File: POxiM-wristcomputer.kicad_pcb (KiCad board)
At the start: 4 copper layers, 38.1 x 22.6 mm, 58 parts, among them J1 USB_B_Micro, J2 AudioJack4_Ground, U1 LM321, U2 STM8S003F3P

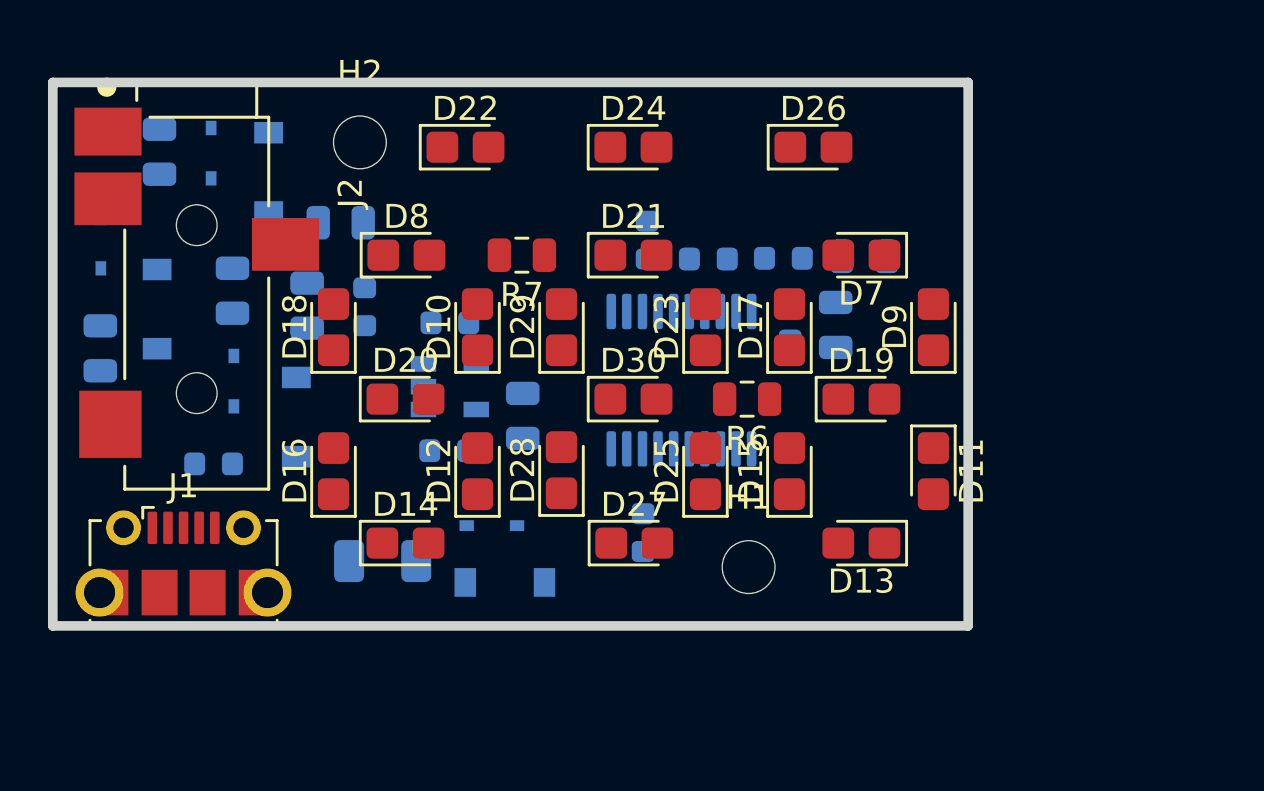
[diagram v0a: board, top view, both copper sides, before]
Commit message: big chungus
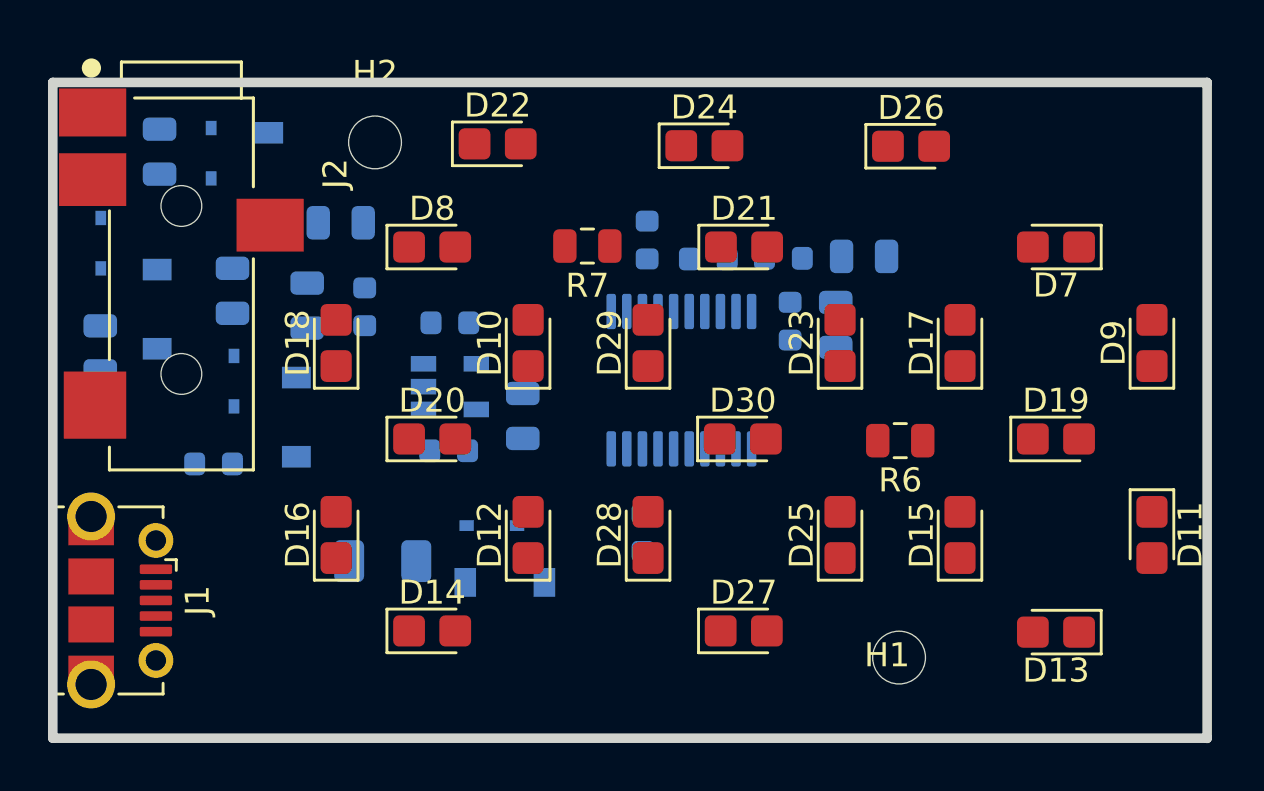
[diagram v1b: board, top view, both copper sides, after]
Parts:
- moved D11 9.49 mm to (117.7, 132.4)
- moved D9 9.13 mm to (117.7, 124.4)
- moved D13 8.92 mm to (113.7, 136.5)
- moved D19 8.28 mm to (113.7, 128.4)
- moved D7 8.12 mm to (113.7, 120.4)
- moved D15 7.59 mm to (109.7, 132.4)
- moved H1 7.32 mm to (107.2, 137.5)
- moved D17 7.14 mm to (109.7, 124.4)
- moved R6 6.61 mm to (107.2, 128.5)
- moved D25 6.21 mm to (104.7, 132.4)
- moved D27 5.85 mm to (100.7, 136.4)
- moved D23 5.65 mm to (104.7, 124.4)
- moved J1 5.44 mm to (72.1, 135.2), turned to 270 degrees
- moved D30 4.85 mm to (100.7, 128.4)
- moved D21 4.62 mm to (100.7, 120.4)
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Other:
- board size 38.1 x 22.6 mm -> 48.1 x 27.3 mm
